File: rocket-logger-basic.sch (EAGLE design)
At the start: 61 parts, among them IC1 CC430F513X, Q2 MOSFET-PCHANNEL, U2 MAX1555, U3 MCP73831, X1 0896BM15A0001, X2 USB-MICROB, X3 SMA-142-0701-801/806

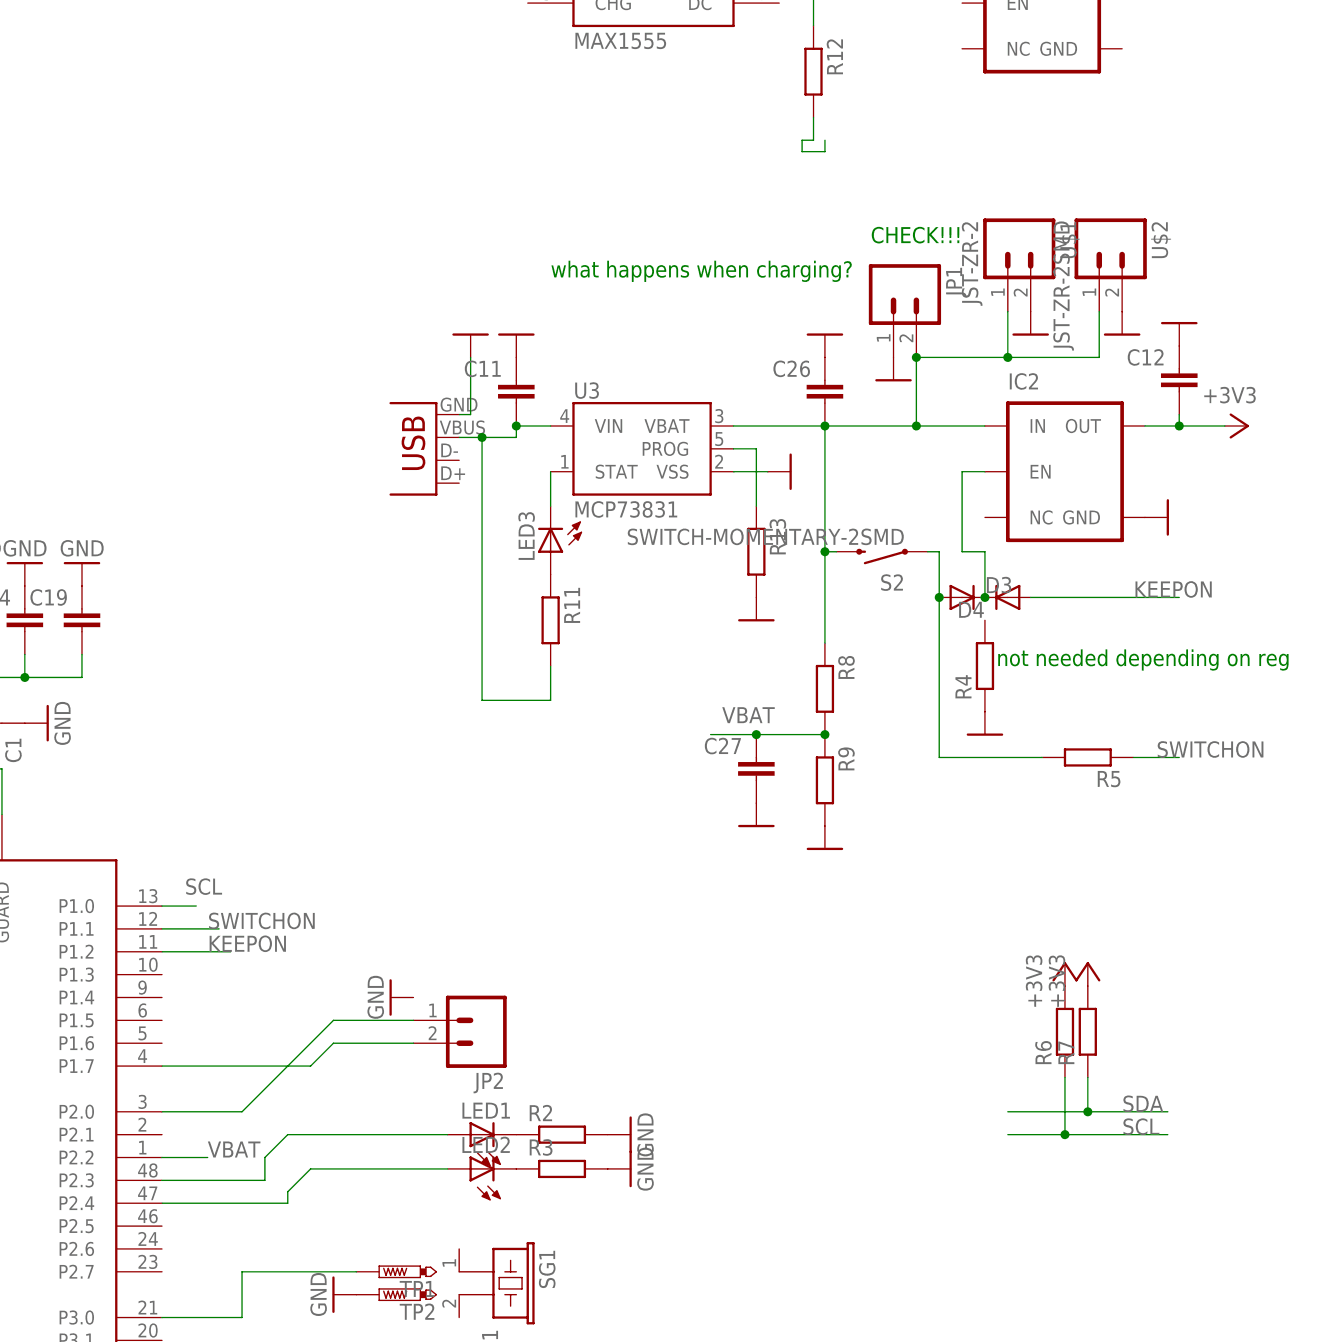
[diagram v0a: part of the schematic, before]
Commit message: basic logger done
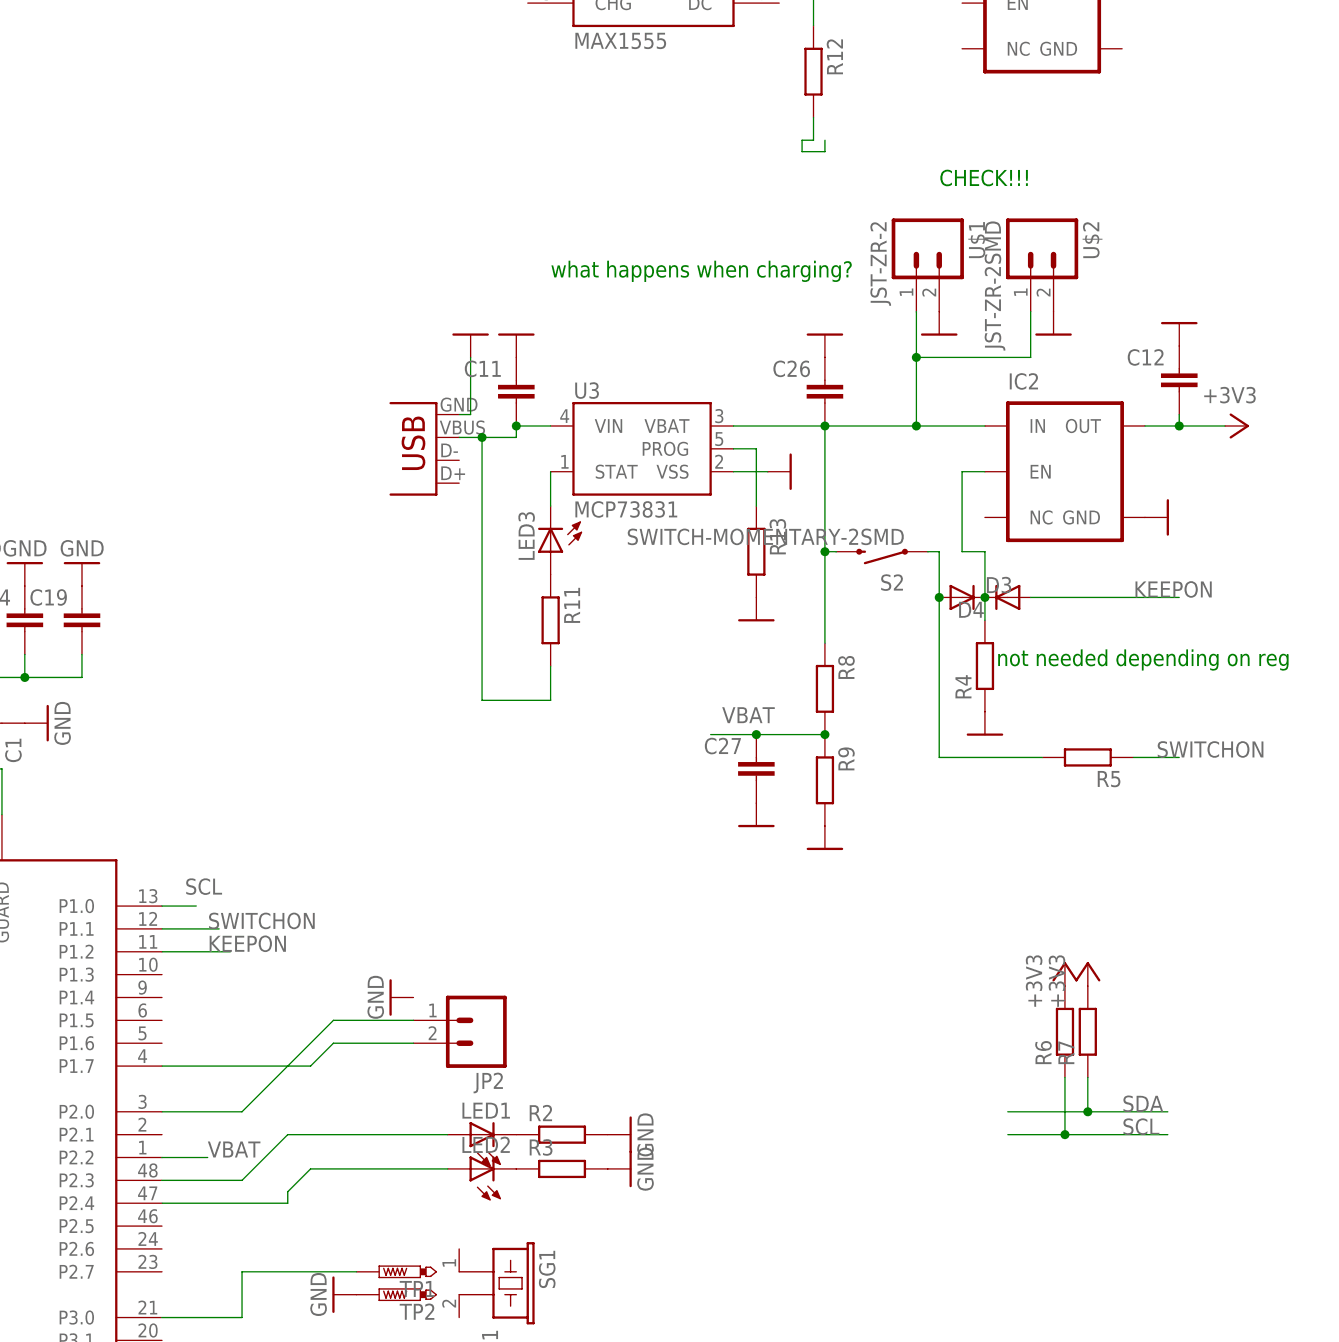
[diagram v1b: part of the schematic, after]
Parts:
- removed JP1: (no value), SparkFun:M02-JST-2MM-SMT
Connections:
- net GND: no longer JP1.1
- net N$2: no longer JP1.2
- net N$25: now also R4.2
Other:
- moved on the sheet: U$1, U$2
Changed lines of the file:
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@@
 <parts>
 <part name="U$4" library="Mine" deviceset="MPL5115A2" device=""/>
-<part name="JP1" library="SparkFun" deviceset="M02" device="-JST-2MM-SMT"/>
 <part name="IC1" library="Mine" deviceset="CC430F513X" device=""/>
 <part name="X1" library="Mine" deviceset="0896BM15A0001" device=""/>
@@
 <part name="C11" library="resistor" deviceset="C-EU" device="C0402"/>
 <part name="GND14" library="SparkFun" deviceset="GND" device=""/>
-<part name="GND15" library="SparkFun" deviceset="GND" device=""/>
 <part name="GND16" library="SparkFun" deviceset="GND" device=""/>
 <part name="+3V1" library="supply1" deviceset="+3V3" device=""/>
@@
 <sheet>
 <plain>
-<text x="144.78" y="248.92" size="1.778" layer="91">CHECK!!!</text>
+<text x="152.4" y="255.27" size="1.778" layer="91">CHECK!!!</text>
 <text x="209.55" y="153.67" size="1.778" layer="91">connect -&gt; ?</text>
 <text x="232.664" y="144.018" size="1.778" layer="91">3</text>
@@
 <instances>
 <instance part="U$4" gate="G$1" x="240.03" y="161.29"/>
-<instance part="JP1" gate="G$1" x="147.32" y="243.84" rot="R270"/>
 <instance part="IC1" gate="G$1" x="53.34" y="160.02"/>
 <instance part="X1" gate="G$1" x="-29.21" y="170.18" rot="MR0"/>
@@
 <instance part="C11" gate="G$1" x="105.41" y="233.68" rot="MR0"/>
 <instance part="GND14" gate="1" x="105.41" y="238.76" smashed="yes" rot="R180"/>
-<instance part="GND15" gate="1" x="147.32" y="233.68" smashed="yes"/>
 <instance part="GND16" gate="1" x="177.8" y="218.44" smashed="yes" rot="R90"/>
 <instance part="+3V1" gate="G$1" x="186.69" y="228.6" rot="R270"/>
@@
 <instance part="Q2" gate="G$1" x="137.16" y="294.64" rot="MR90"/>
 <instance part="R12" gate="G$1" x="138.43" y="267.97" rot="R270"/>
-<instance part="U$1" gate="G$1" x="160.02" y="248.92" rot="R270"/>
-<instance part="U$2" gate="G$1" x="170.18" y="248.92" rot="R270"/>
-<instance part="GND31" gate="1" x="172.72" y="238.76" smashed="yes"/>
-<instance part="GND33" gate="1" x="162.56" y="238.76" smashed="yes"/>
+<instance part="U$1" gate="G$1" x="149.86" y="248.92" rot="R270"/>
+<instance part="U$2" gate="G$1" x="162.56" y="248.92" rot="R270"/>
+<instance part="GND31" gate="1" x="165.1" y="238.76" smashed="yes"/>
+<instance part="GND33" gate="1" x="152.4" y="238.76" smashed="yes"/>
 <instance part="U3" gate="G$1" x="119.38" y="226.06"/>
 <instance part="R13" gate="G$1" x="132.08" y="214.63" rot="R270"/>
@@
 </segment>
 <segment>
-<pinref part="JP1" gate="G$1" pin="1"/>
-<pinref part="GND15" gate="1" pin="GND"/>
-</segment>
-<segment>
 <pinref part="IC2" gate="G$1" pin="GND"/>
 <pinref part="GND16" gate="1" pin="GND"/>
@@
 <net name="N$2" class="0">
 <segment>
-<pinref part="JP1" gate="G$1" pin="2"/>
 <wire x1="139.7" y1="228.6" x2="149.86" y2="228.6" width="0.1524" layer="91"/>
 <wire x1="149.86" y1="236.22" x2="149.86" y2="228.6" width="0.1524" layer="91"/>
@@
 <pinref part="U$2" gate="G$1" pin="1"/>
 <wire x1="139.7" y1="214.63" x2="139.7" y2="228.6" width="0.1524" layer="91"/>
-<wire x1="170.18" y1="241.3" x2="170.18" y2="236.22" width="0.1524" layer="91"/>
-<wire x1="170.18" y1="236.22" x2="160.02" y2="236.22" width="0.1524" layer="91"/>
+<wire x1="162.56" y1="241.3" x2="162.56" y2="236.22" width="0.1524" layer="91"/>
+<wire x1="162.56" y1="236.22" x2="149.86" y2="236.22" width="0.1524" layer="91"/>
 <pinref part="U$1" gate="G$1" pin="1"/>
-<wire x1="160.02" y1="236.22" x2="149.86" y2="236.22" width="0.1524" layer="91"/>
-<wire x1="160.02" y1="241.3" x2="160.02" y2="236.22" width="0.1524" layer="91"/>
+<wire x1="149.86" y1="241.3" x2="149.86" y2="236.22" width="0.1524" layer="91"/>
 <junction x="149.86" y="236.22"/>
-<junction x="160.02" y="236.22"/>
 <pinref part="U3" gate="G$1" pin="VBAT"/>
 <wire x1="129.54" y1="228.6" x2="139.7" y2="228.6" width="0.1524" layer="91"/>
@@
 <net name="N$16" class="0">
 <segment>
-<wire x1="80.01" y1="149.86" x2="77.47" y2="147.32" width="0.1524" layer="91"/>
 <pinref part="IC1" gate="G$1" pin="P2.3"/>
-<wire x1="66.04" y1="144.78" x2="77.47" y2="144.78" width="0.1524" layer="91"/>
-<wire x1="77.47" y1="144.78" x2="77.47" y2="147.32" width="0.1524" layer="91"/>
+<wire x1="66.04" y1="144.78" x2="74.93" y2="144.78" width="0.1524" layer="91"/>
+<wire x1="74.93" y1="144.78" x2="80.01" y2="149.86" width="0.1524" layer="91"/>
 <pinref part="LED1" gate="G$1" pin="A"/>
 <wire x1="97.79" y1="149.86" x2="80.01" y2="149.86" width="0.1524" layer="91"/>
@@
 <wire x1="154.94" y1="214.63" x2="154.94" y2="223.52" width="0.1524" layer="91"/>
 <junction x="157.48" y="209.55"/>
-</segment>
-</net>
+<pinref part="R4" gate="G$1" pin="2"/>
+<wire x1="157.48" y1="207.01" x2="157.48" y2="209.55" width="0.1524" layer="91"/>
+</segment>
+</net>
